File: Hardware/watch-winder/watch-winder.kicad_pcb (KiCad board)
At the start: 4 copper layers, 50 x 35 mm, 56 parts, among them J1 SWD, J2 UART, J3 MOT, J4 SYNC0, J5 SYNC1, J6 PWR, SW1 SW_Push, SW2 SW_Push, SW3 SW_Push, U1 STM32F030K6Tx, U2 M24C02-FMN, U3 ULN2003, U4 AMS1117-3.3, Y1 8M

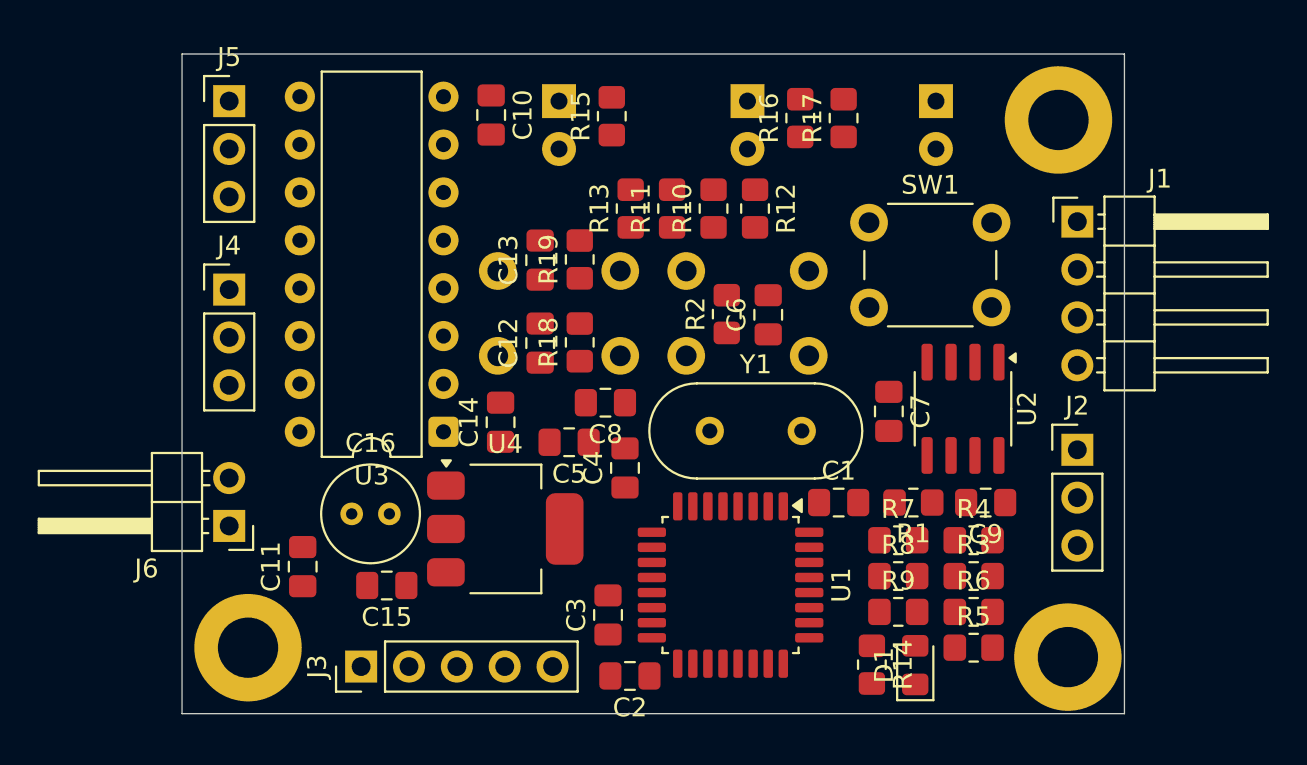
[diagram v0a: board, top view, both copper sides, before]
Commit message: routing
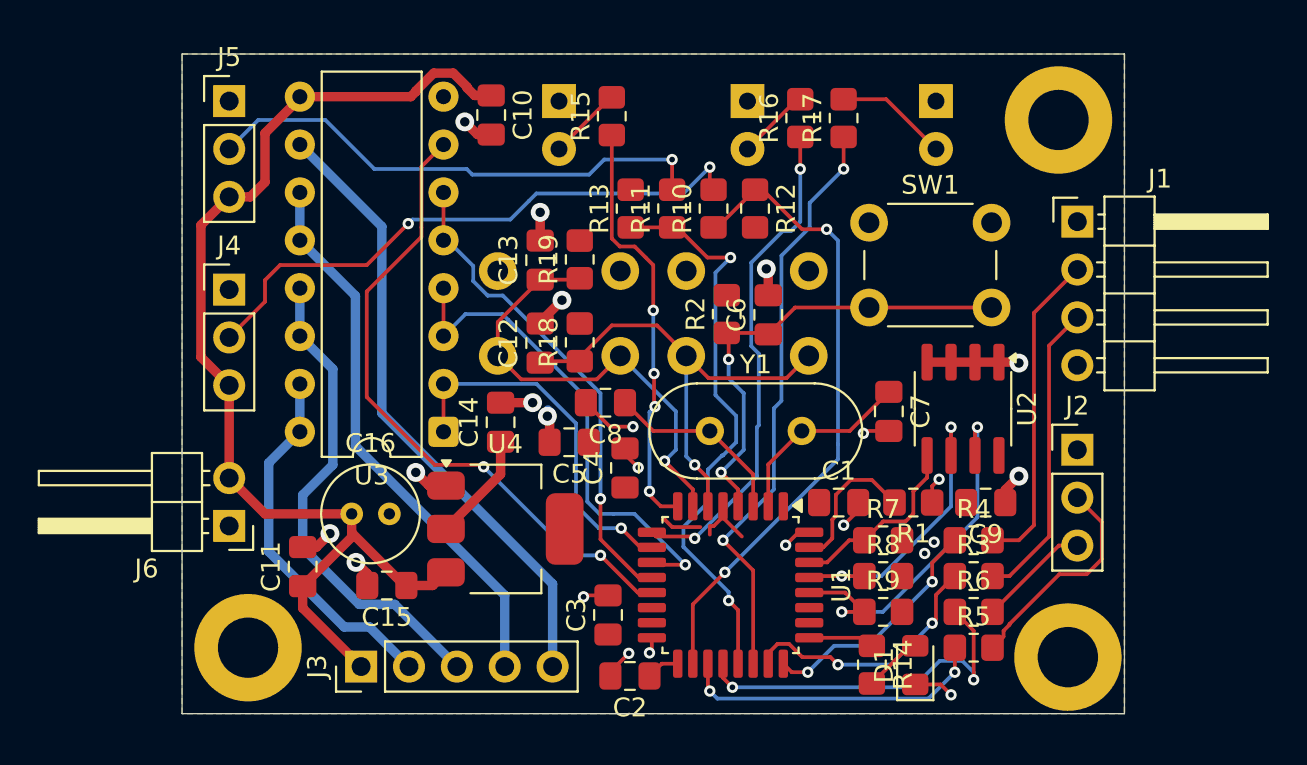
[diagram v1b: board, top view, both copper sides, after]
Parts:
- moved R7 0.80 mm to (197.2, 140.8)
- moved R8 0.80 mm to (197.2, 142.7)
- moved R9 0.80 mm to (197.2, 144.6)
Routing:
- net +5V: track 0.00 -> 59.1 mm
- net GND: track 0.00 -> 37.7 mm, vias 0 -> 21
- net /MOT3: track 0.00 -> 34.5 mm, vias 0 -> 2
- net /SYNC0: track 0.00 -> 34.2 mm, vias 0 -> 2
- net Net-(J3-Pin_5): track 0.00 -> 33.2 mm
- net /LED2: track 0.00 -> 31.3 mm, vias 0 -> 2
- net Net-(J4-Pin_2): track 0.00 -> 31.2 mm, vias 0 -> 2
- net /SYNC1: track 0.00 -> 30.7 mm, vias 0 -> 2
- net Net-(J3-Pin_4): track 0.00 -> 29.7 mm
- net Net-(J5-Pin_2): track 0.00 -> 27.3 mm, vias 0 -> 1
- net /LED1: track 0.00 -> 26.6 mm, vias 0 -> 2
- net /MOT1: track 0.00 -> 26.4 mm, vias 0 -> 1
- net /MOT2: track 0.00 -> 26.0 mm, vias 0 -> 1
- net Net-(J3-Pin_3): track 0.00 -> 26.0 mm
- net /BUT0: track 0.00 -> 25.3 mm, vias 0 -> 1
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- added copper zone on B.Cu, net +3V3
- added copper zone on F.Cu, net +3V3
